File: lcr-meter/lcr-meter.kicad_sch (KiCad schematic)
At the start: 0 parts

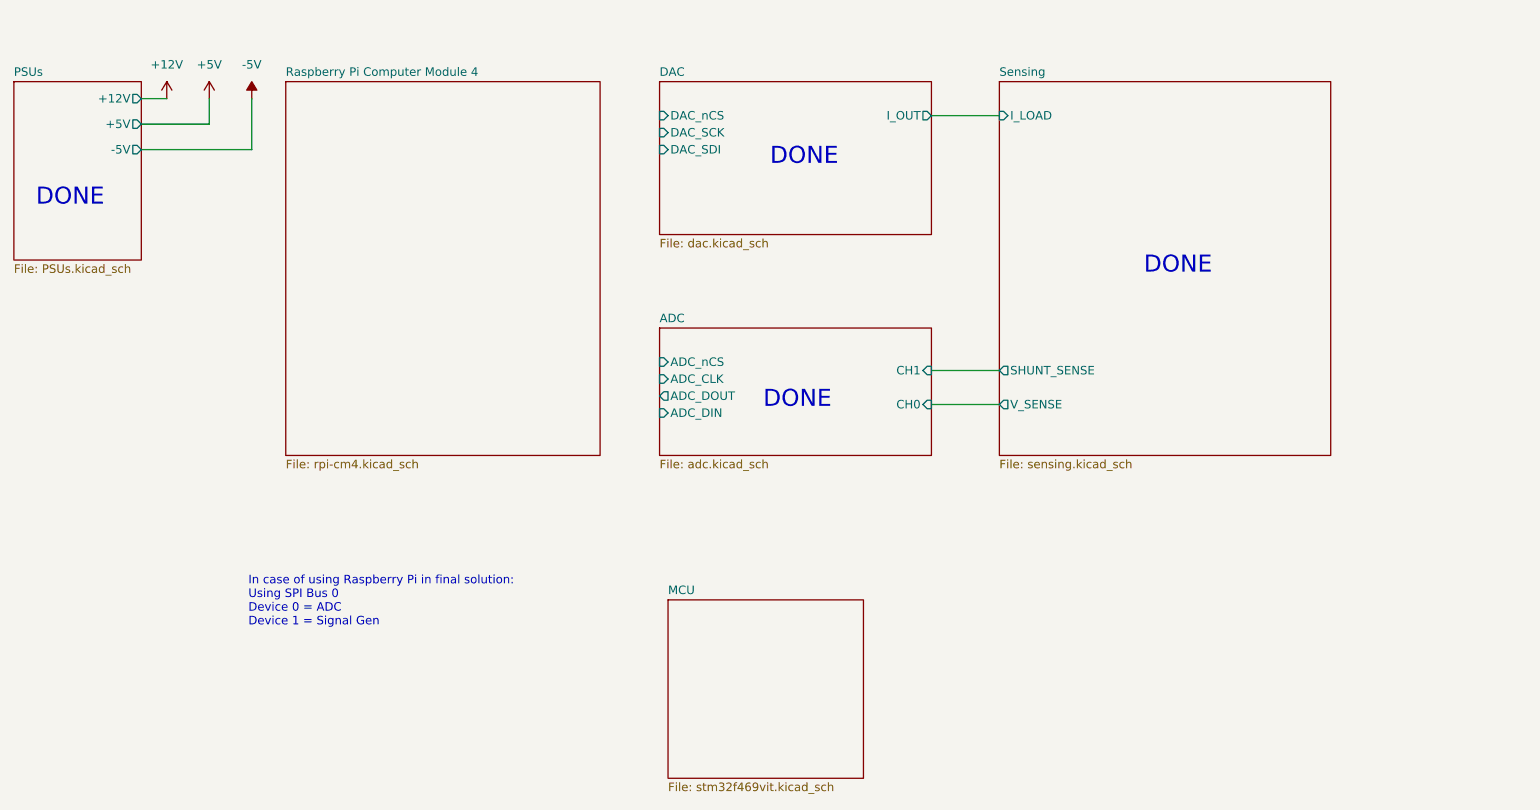
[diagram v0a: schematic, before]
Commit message: Schematic completion
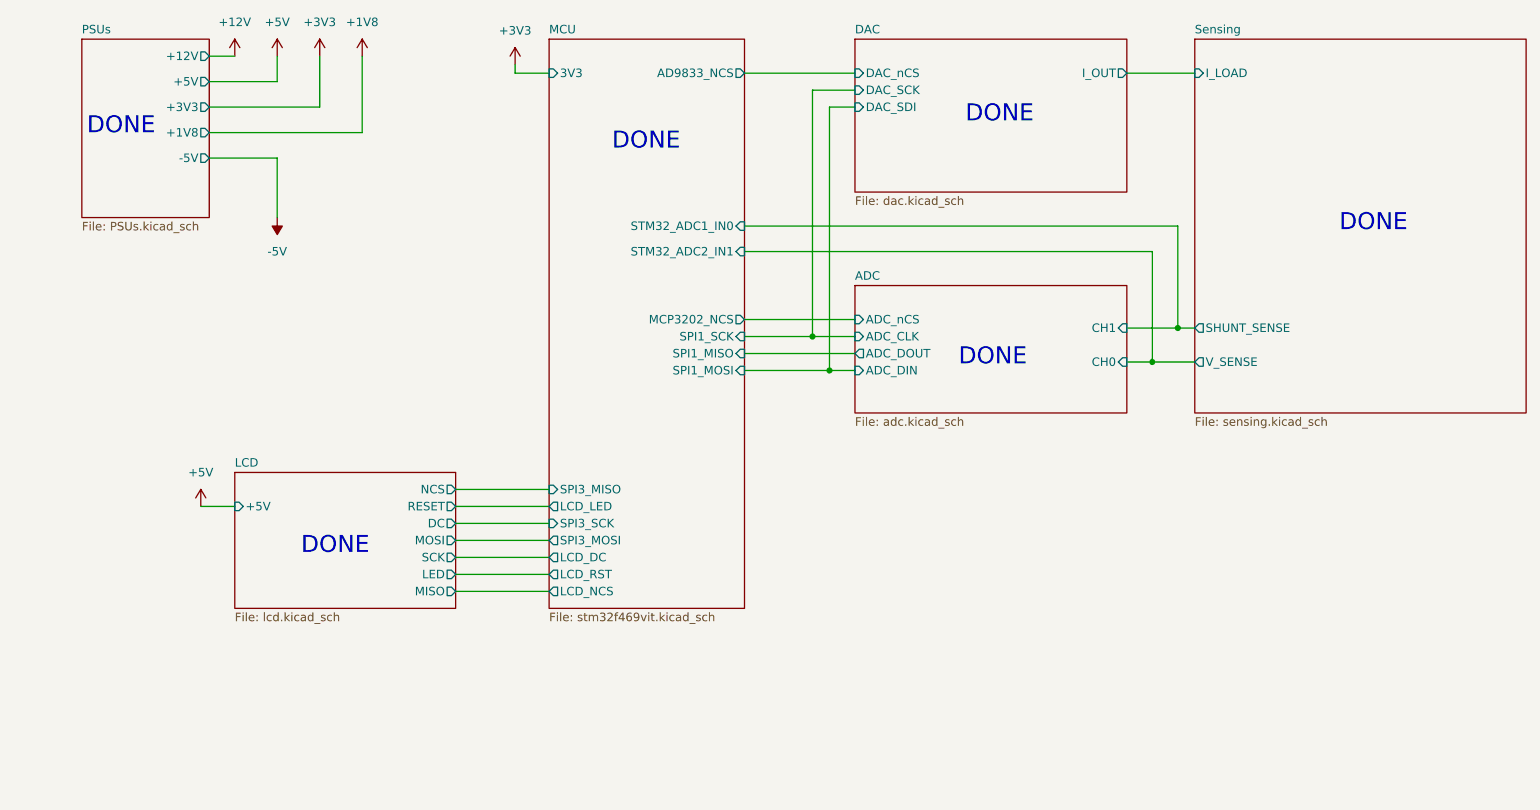
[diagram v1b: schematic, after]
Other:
- removed sheet Raspberry Pi Computer Module 4
- added sheet LCD (lcd.kicad_sch)
- sheet MCU ports: added 3V3, AD9833_NCS, LCD_DC, LCD_LED, LCD_NCS, LCD_RST, MCP3202_NCS, SPI1_MISO, SPI1_MOSI, SPI1_SCK, SPI3_MISO, SPI3_MOSI, SPI3_SCK, STM32_ADC1_IN0, STM32_ADC2_IN1; removed none
- sheet PSUs ports: added +1V8, +3V3; removed none
- note removed: "In case of using Raspberry Pi in final solution: Using SPI Bus 0 Device 0 = ADC Device 1 = Signal Gen"

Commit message: Schematic polishing
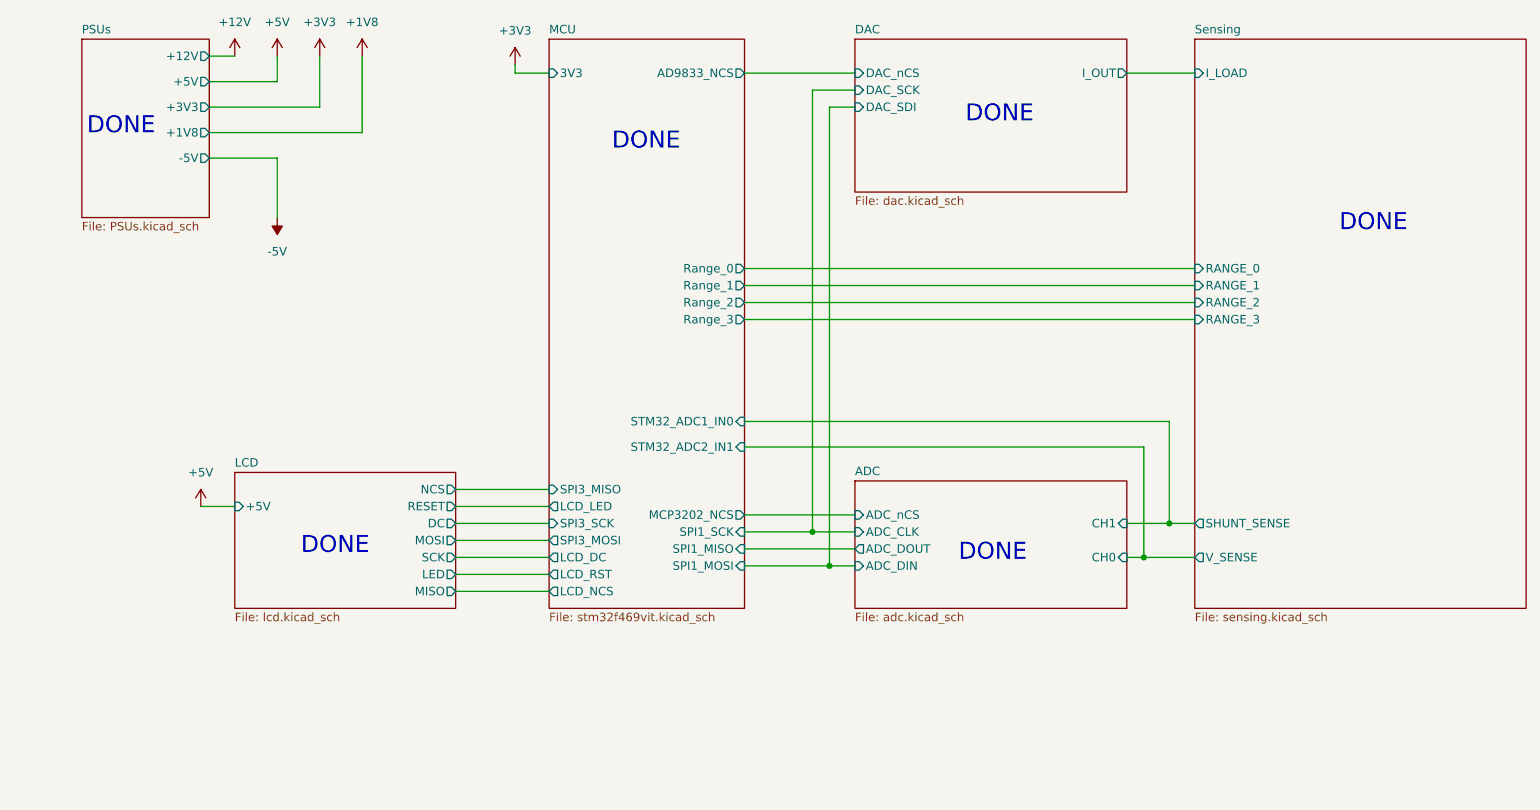
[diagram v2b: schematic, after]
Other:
- sheet MCU ports: added Range_0, Range_1, Range_2, Range_3; removed none
- sheet Sensing ports: added RANGE_0, RANGE_1, RANGE_2, RANGE_3; removed none
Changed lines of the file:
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@@
 	(paper "A4")
 	(junction
-		(at 196.85 102.87)
+		(at 195.58 132.08)
 		(diameter 0)
 		(color 0 0 0 0)
 	)
 	(junction
-		(at 193.04 107.95)
+		(at 142.24 133.35)
 		(diameter 0)
 		(color 0 0 0 0)
 	)
 	(junction
-		(at 142.24 104.14)
+		(at 191.77 137.16)
 		(diameter 0)
 		(color 0 0 0 0)
 	)
 	(junction
-		(at 144.78 109.22)
+		(at 144.78 138.43)
 		(diameter 0)
 		(color 0 0 0 0)
@@
 	(wire
 		(pts
-			(xy 193.04 91.44) (xy 193.04 107.95)
-		)
-		(stroke
-			(width 0)
-			(type default)
-		)
-	)
-	(wire
-		(pts
-			(xy 132.08 101.6) (xy 148.59 101.6)
+			(xy 132.08 99.06) (xy 199.39 99.06)
+		)
+		(stroke
+			(width 0)
+			(type default)
+		)
+	)
+	(wire
+		(pts
+			(xy 191.77 120.65) (xy 191.77 137.16)
+		)
+		(stroke
+			(width 0)
+			(type default)
+		)
+	)
+	(wire
+		(pts
+			(xy 142.24 67.31) (xy 142.24 133.35)
+		)
+		(stroke
+			(width 0)
+			(type default)
+		)
+	)
+	(wire
+		(pts
+			(xy 132.08 130.81) (xy 148.59 130.81)
 		)
 		(stroke
@@
 	(wire
 		(pts
-			(xy 189.23 102.87) (xy 196.85 102.87)
+			(xy 189.23 132.08) (xy 195.58 132.08)
 		)
 		(stroke
@@
 	(wire
 		(pts
-			(xy 142.24 104.14) (xy 148.59 104.14)
-		)
-		(stroke
-			(width 0)
-			(type default)
-		)
-	)
-	(wire
-		(pts
-			(xy 193.04 107.95) (xy 199.39 107.95)
+			(xy 132.08 93.98) (xy 199.39 93.98)
+		)
+		(stroke
+			(width 0)
+			(type default)
+		)
+	)
+	(wire
+		(pts
+			(xy 142.24 133.35) (xy 148.59 133.35)
 		)
 		(stroke
@@
 	(wire
 		(pts
-			(xy 132.08 87.63) (xy 196.85 87.63)
+			(xy 132.08 116.84) (xy 195.58 116.84)
 		)
 		(stroke
@@
 	(wire
 		(pts
-			(xy 144.78 109.22) (xy 148.59 109.22)
-		)
-		(stroke
-			(width 0)
-			(type default)
-		)
-	)
-	(wire
-		(pts
-			(xy 196.85 102.87) (xy 199.39 102.87)
+			(xy 144.78 138.43) (xy 148.59 138.43)
+		)
+		(stroke
+			(width 0)
+			(type default)
+		)
+	)
+	(wire
+		(pts
+			(xy 132.08 101.6) (xy 199.39 101.6)
 		)
 		(stroke
@@
 	(wire
 		(pts
-			(xy 144.78 69.85) (xy 144.78 109.22)
-		)
-		(stroke
-			(width 0)
-			(type default)
-		)
-	)
-	(wire
-		(pts
-			(xy 132.08 91.44) (xy 193.04 91.44)
+			(xy 132.08 120.65) (xy 191.77 120.65)
 		)
 		(stroke
@@
 	(wire
 		(pts
+			(xy 195.58 132.08) (xy 199.39 132.08)
+		)
+		(stroke
+			(width 0)
+			(type default)
+		)
+	)
+	(wire
+		(pts
+			(xy 191.77 137.16) (xy 199.39 137.16)
+		)
+		(stroke
+			(width 0)
+			(type default)
+		)
+	)
+	(wire
+		(pts
 			(xy 88.9 134.62) (xy 102.87 134.62)
 		)
@@
 	(wire
 		(pts
-			(xy 142.24 67.31) (xy 142.24 104.14)
-		)
-		(stroke
-			(width 0)
-			(type default)
-		)
-	)
-	(wire
-		(pts
 			(xy 148.59 69.85) (xy 144.78 69.85)
 		)
@@
 	(wire
 		(pts
-			(xy 132.08 106.68) (xy 148.59 106.68)
+			(xy 144.78 69.85) (xy 144.78 138.43)
+		)
+		(stroke
+			(width 0)
+			(type default)
+		)
+	)
+	(wire
+		(pts
+			(xy 132.08 135.89) (xy 148.59 135.89)
 		)
 		(stroke
@@
 	(wire
 		(pts
-			(xy 189.23 107.95) (xy 193.04 107.95)
+			(xy 189.23 137.16) (xy 191.77 137.16)
 		)
 		(stroke
@@
 	(wire
 		(pts
-			(xy 132.08 104.14) (xy 142.24 104.14)
+			(xy 132.08 133.35) (xy 142.24 133.35)
 		)
 		(stroke
@@
 	(wire
 		(pts
+			(xy 132.08 96.52) (xy 199.39 96.52)
+		)
+		(stroke
+			(width 0)
+			(type default)
+		)
+	)
+	(wire
+		(pts
 			(xy 68.58 62.23) (xy 68.58 69.85)
 		)
@@
 	(wire
 		(pts
-			(xy 132.08 109.22) (xy 144.78 109.22)
-		)
-		(stroke
-			(width 0)
-			(type default)
-		)
-	)
-	(wire
-		(pts
-			(xy 196.85 87.63) (xy 196.85 102.87)
+			(xy 132.08 138.43) (xy 144.78 138.43)
+		)
+		(stroke
+			(width 0)
+			(type default)
+		)
+	)
+	(wire
+		(pts
+			(xy 195.58 116.84) (xy 195.58 132.08)
 		)
 		(stroke
@@
 	(text "DONE"
 		(exclude_from_sim no)
-		(at 164.084 108.712 0)
+		(at 164.084 137.922 0)
 		(effects
 			(font
@@
 		)
 		(pin "SPI1_MISO" input
-			(at 132.08 106.68 0)
+			(at 132.08 135.89 0)
 			(effects
 				(font
@@
 		)
 		(pin "SPI1_MOSI" input
-			(at 132.08 109.22 0)
+			(at 132.08 138.43 0)
 			(effects
 				(font
@@
 		)
 		(pin "SPI1_SCK" input
-			(at 132.08 104.14 0)
+			(at 132.08 133.35 0)
 			(effects
 				(font
@@
 		)
 		(pin "STM32_ADC2_IN1" input
-			(at 132.08 91.44 0)
+			(at 132.08 120.65 0)
 			(effects
 				(font
@@
 		)
 		(pin "STM32_ADC1_IN0" input
-			(at 132.08 87.63 0)
+			(at 132.08 116.84 0)
 			(effects
 				(font
@@
 		)
 		(pin "MCP3202_NCS" output
+			(at 132.08 130.81 0)
+			(effects
+				(font
+					(size 1.27 1.27)
+				)
+				(justify right)
+			)
+		)
+		(pin "Range_0" output
+			(at 132.08 93.98 0)
+			(effects
+				(font
+					(size 1.27 1.27)
+				)
+				(justify right)
+			)
+		)
+		(pin "Range_1" output
+			(at 132.08 96.52 0)
+			(effects
+				(font
+					(size 1.27 1.27)
+				)
+				(justify right)
+			)
+		)
+		(pin "Range_2" output
+			(at 132.08 99.06 0)
+			(effects
+				(font
+					(size 1.27 1.27)
+				)
+				(justify right)
+			)
+		)
+		(pin "Range_3" output
 			(at 132.08 101.6 0)
 			(effects
@@
 	(sheet
 		(at 199.39 59.69)
-		(size 49.53 55.88)
+		(size 49.53 85.09)
 		(fields_autoplaced yes)
 		(stroke
@@
 		)
 		(property "Sheetfile" "sensing.kicad_sch"
-			(at 199.39 116.1546 0)
+			(at 199.39 145.3646 0)
 			(effects
 				(font
@@
 		)
 		(pin "SHUNT_SENSE" output
-			(at 199.39 102.87 180)
+			(at 199.39 132.08 180)
 			(effects
 				(font
@@
 		)
 		(pin "V_SENSE" output
-			(at 199.39 107.95 180)
+			(at 199.39 137.16 180)
 			(effects
 				(font
@@
 		(pin "I_LOAD" input
 			(at 199.39 64.77 180)
+			(effects
+				(font
+					(size 1.27 1.27)
+				)
+				(justify left)
+			)
+		)
+		(pin "RANGE_0" input
+			(at 199.39 93.98 180)
+			(effects
+				(font
+					(size 1.27 1.27)
+				)
+				(justify left)
+			)
+		)
+		(pin "RANGE_1" input
+			(at 199.39 96.52 180)
+			(effects
+				(font
+					(size 1.27 1.27)
+				)
+				(justify left)
+			)
+		)
+		(pin "RANGE_2" input
+			(at 199.39 99.06 180)
+			(effects
+				(font
+					(size 1.27 1.27)
+				)
+				(justify left)
+			)
+		)
+		(pin "RANGE_3" input
+			(at 199.39 101.6 180)
 			(effects
 				(font
@@
 	)
 	(sheet
-		(at 148.59 96.52)
+		(at 148.59 125.73)
 		(size 40.64 19.05)
 		(fields_autoplaced yes)
@@
 		)
 		(property "Sheetname" "ADC"
-			(at 148.59 95.8084 0)
+			(at 148.59 125.0184 0)
 			(effects
 				(font
@@
 		)
 		(property "Sheetfile" "adc.kicad_sch"
-			(at 148.59 116.1546 0)
+			(at 148.59 145.3646 0)
 			(effects
 				(font
@@
 		)
 		(pin "CH1" input
-			(at 189.23 102.87 0)
+			(at 189.23 132.08 0)
 			(effects
 				(font
@@
 		)
 		(pin "CH0" input
-			(at 189.23 107.95 0)
+			(at 189.23 137.16 0)
 			(effects
 				(font
@@
 		)
 		(pin "ADC_nCS" input
-			(at 148.59 101.6 180)
+			(at 148.59 130.81 180)
 			(effects
 				(font
@@
 		)
 		(pin "ADC_CLK" input
-			(at 148.59 104.14 180)
+			(at 148.59 133.35 180)
 			(effects
 				(font
@@
 		)
 		(pin "ADC_DOUT" output
-			(at 148.59 106.68 180)
+			(at 148.59 135.89 180)
 			(effects
 				(font
@@
 		)
 		(pin "ADC_DIN" input
-			(at 148.59 109.22 180)
-			(effects
-				(font
+			(at 148.59 138.43 180)
+			(effects
+				(font
